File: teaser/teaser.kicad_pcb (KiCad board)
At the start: 2 copper layers, 71 parts, among them J1 Programator, J2 AC_Plug, J3 OLED, J4 battery, Q1 MMBTA44, Q2 MMBTA44, Q3 MMBTA44, Q4 MMBTA44, Q6 AO3401A, SW1 Włancznik, SW2 SW_SPST, SW3 Manual, SW4 Manual, SW5 Manual, SW7 SW_Push, U2 LM1117MP-5.0, U3 ATmega328P-A, Y1 16kHz

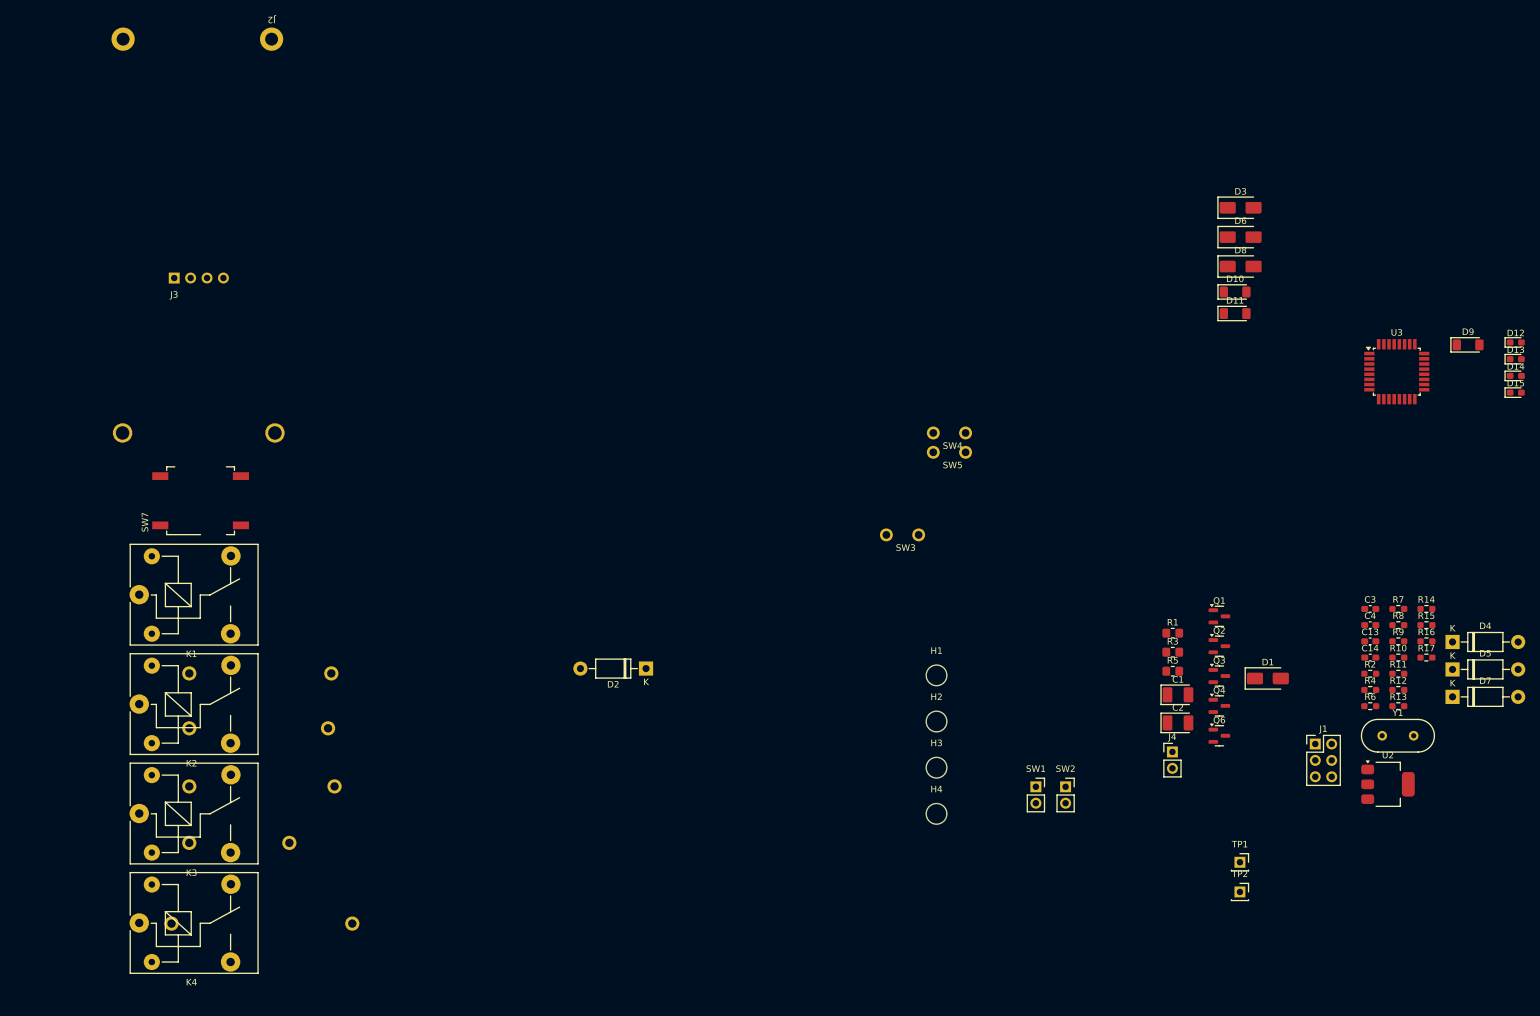
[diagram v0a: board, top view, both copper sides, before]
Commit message: Most of high voltage routed
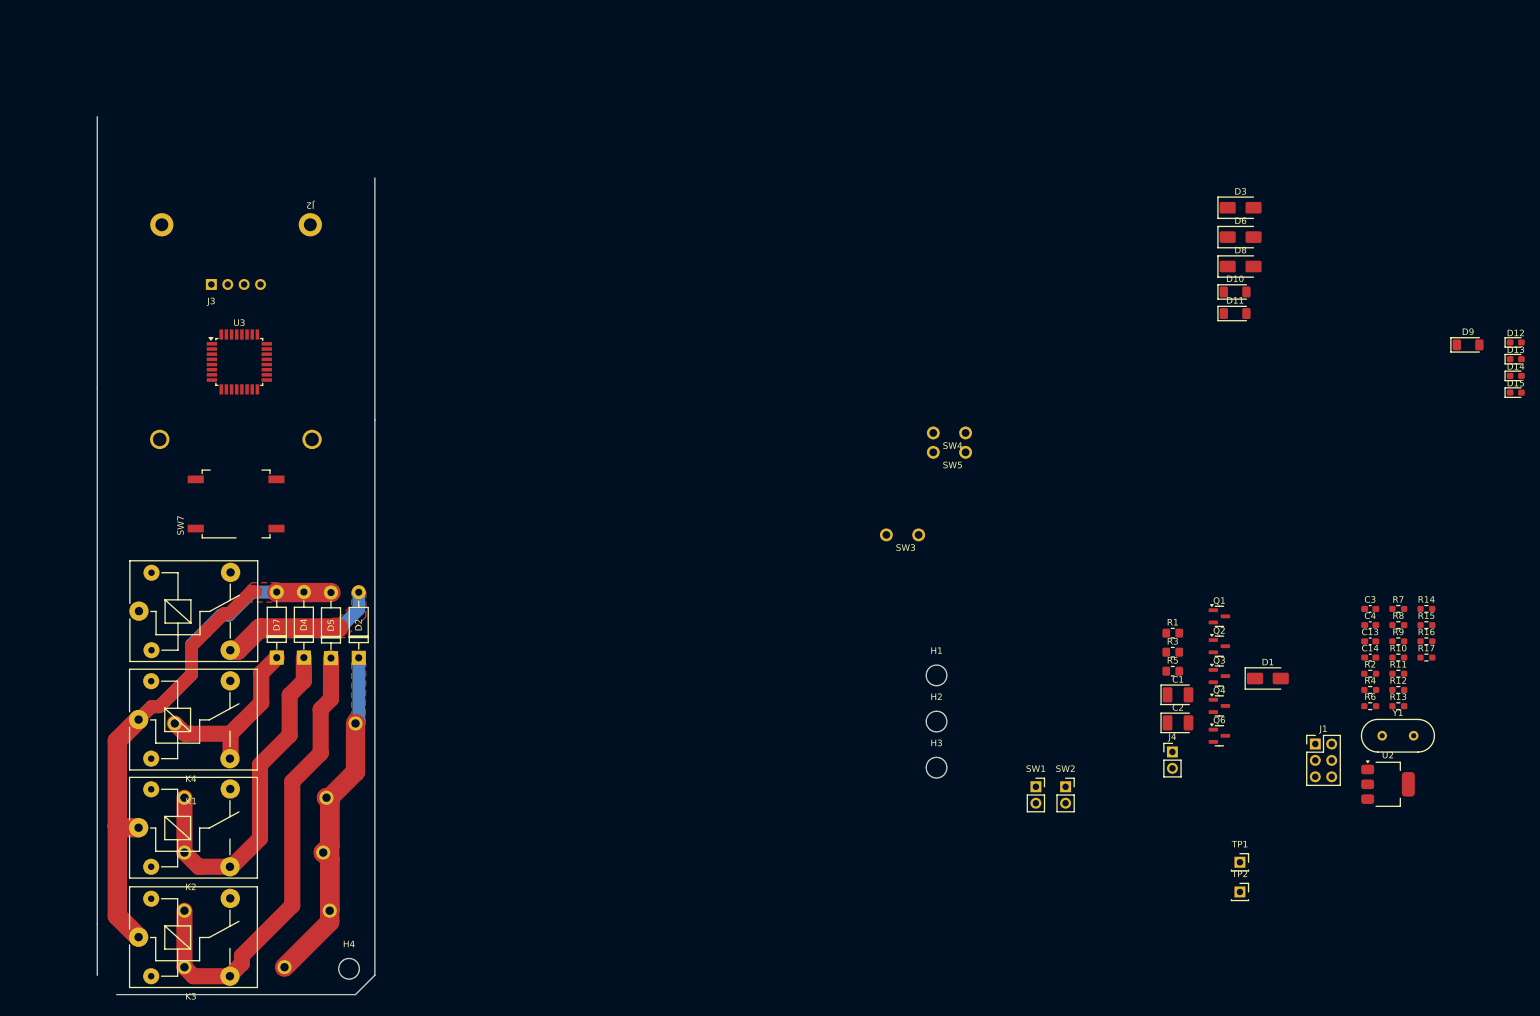
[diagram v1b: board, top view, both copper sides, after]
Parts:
- moved D7 182.2 mm to (78.8, 128.8), turned to 90 degrees
- moved U3 179.3 mm to (73.0, 83.0)
- moved D4 177.9 mm to (83.0, 128.8), turned to 90 degrees
- moved D5 173.7 mm to (87.2, 128.9), turned to 90 degrees
- moved H4 94.1 mm to (90.0, 177.0)
- moved D2 44.5 mm to (91.5, 128.8), turned to 90 degrees
- moved C12 42.1 mm to (91.0, 139.0), turned to 180 degrees
- moved K4 31.5 mm to (57.4, 138.4)
- moved J2 29.4 mm to (84.0, 61.8)
- moved C11 29.0 mm to (87.0, 168.0), turned to 180 degrees
- moved C8 28.7 mm to (86.5, 150.5), turned to 180 degrees
- moved C7 28.3 mm to (86.0, 159.0), turned to 180 degrees
- moved C10 24.3 mm to (80.0, 176.8), turned to 180 degrees
- moved K2 19.2 mm to (57.4, 155.2)
- moved K3 19.2 mm to (57.4, 172.1)
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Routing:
- net Net-(D4-A): track 0.00 -> 109.7 mm
- net /CH2_230: track 0.00 -> 72.1 mm
- net Net-(D2-K): track 0.00 -> 71.2 mm
- net /CH3_230: track 0.00 -> 53.8 mm
- net Net-(D2-A): track 0.00 -> 43.0 mm
- net /CH1_230: track 0.00 -> 30.2 mm
- added copper zone on F.Cu, net Net-(D2-A)
- added copper zone on F.Cu, net Net-(D2-K)
- added copper zone on F.Cu, net Net-(D4-A)
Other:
- board outline added: 43 x 136 mm

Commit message: Continue routing
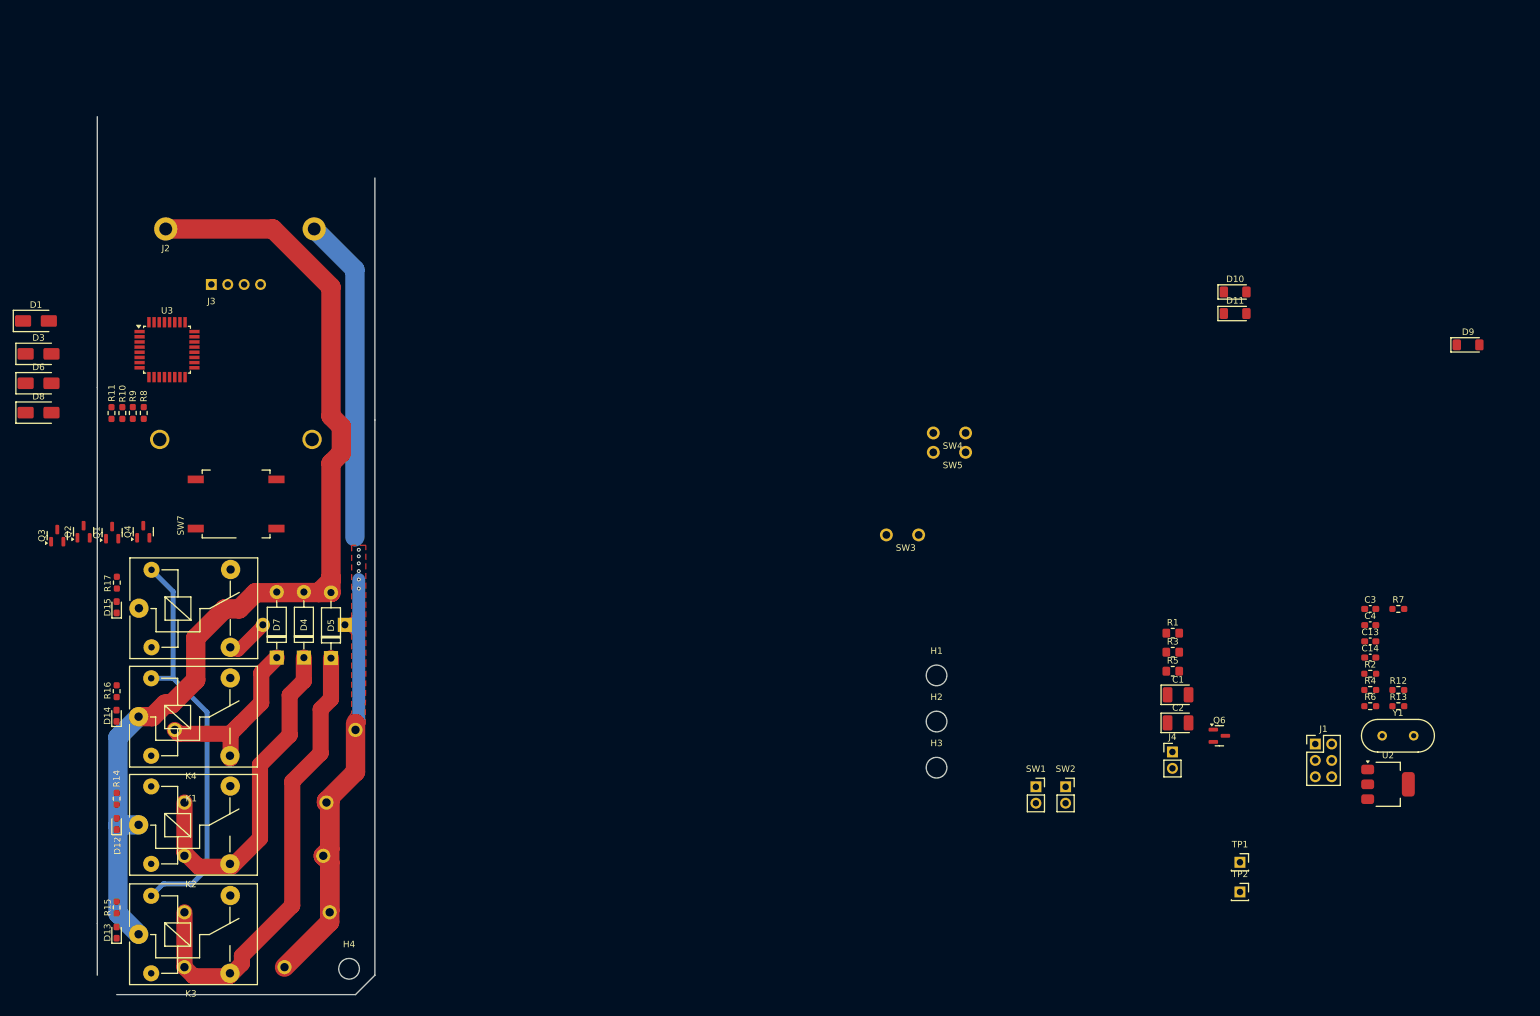
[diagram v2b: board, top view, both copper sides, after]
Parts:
- D2: footprint Diode_THT:D_DO-41_SOD81_P10.16mm_Horizontal -> Diode_THT:D_DO-41_SOD81_P12.70mm_Horizontal; moved to B.Cu
- moved D13 234.2 mm to (54.0, 171.4), turned to 90 degrees
- moved D12 229.2 mm to (54.0, 154.6), turned to 90 degrees
- moved D14 223.0 mm to (54.0, 137.8), turned to 90 degrees
- moved D15 219.3 mm to (54.0, 121.0), turned to 90 degrees
- moved R15 207.5 mm to (54.0, 167.5), turned to -90 degrees
- moved R14 205.0 mm to (54.0, 150.7), turned to -90 degrees
- moved R11 203.4 mm to (53.2, 90.9), turned to 90 degrees
- moved R17 203.2 mm to (54.0, 117.2), turned to -90 degrees
- moved R16 203.0 mm to (54.0, 134.0), turned to -90 degrees
- moved R10 201.2 mm to (54.9, 90.9), turned to 90 degrees
- moved R9 199.2 mm to (56.5, 90.9), turned to 90 degrees
- moved D1 198.7 mm to (41.5, 76.7)
- moved R8 197.1 mm to (58.2, 90.9), turned to 90 degrees
- moved D3 187.6 mm to (41.9, 81.8)
- moved D6 187.6 mm to (41.9, 86.3)
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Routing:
- net Net-(D2-K): track 71.2 -> 139.1 mm, vias 0 -> 6
- net VCC: track 0.00 -> 64.7 mm
- net Net-(D4-A): track 109.7 -> 162.0 mm
- net Net-(D2-A): track 43.0 -> 6.75 mm
- net /CH3_230: track 53.8 -> 53.0 mm
- removed copper zone on F.Cu, net Net-(D2-A)
- removed copper zone on F.Cu, net Net-(D4-A)
